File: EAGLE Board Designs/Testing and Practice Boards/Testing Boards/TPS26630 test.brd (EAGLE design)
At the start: 100 x 80 mm, 3 parts

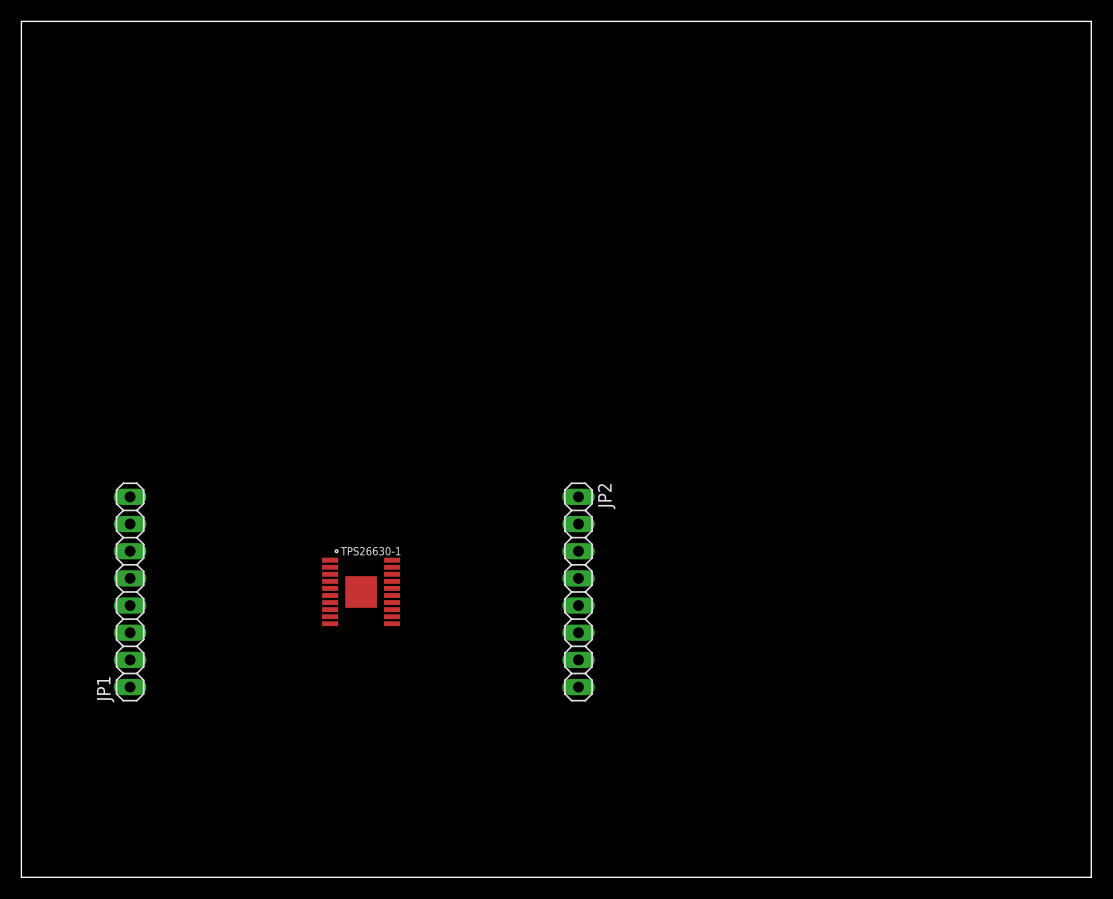
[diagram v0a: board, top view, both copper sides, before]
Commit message: Finished the TPS26630 E-Fuse breakout board layout
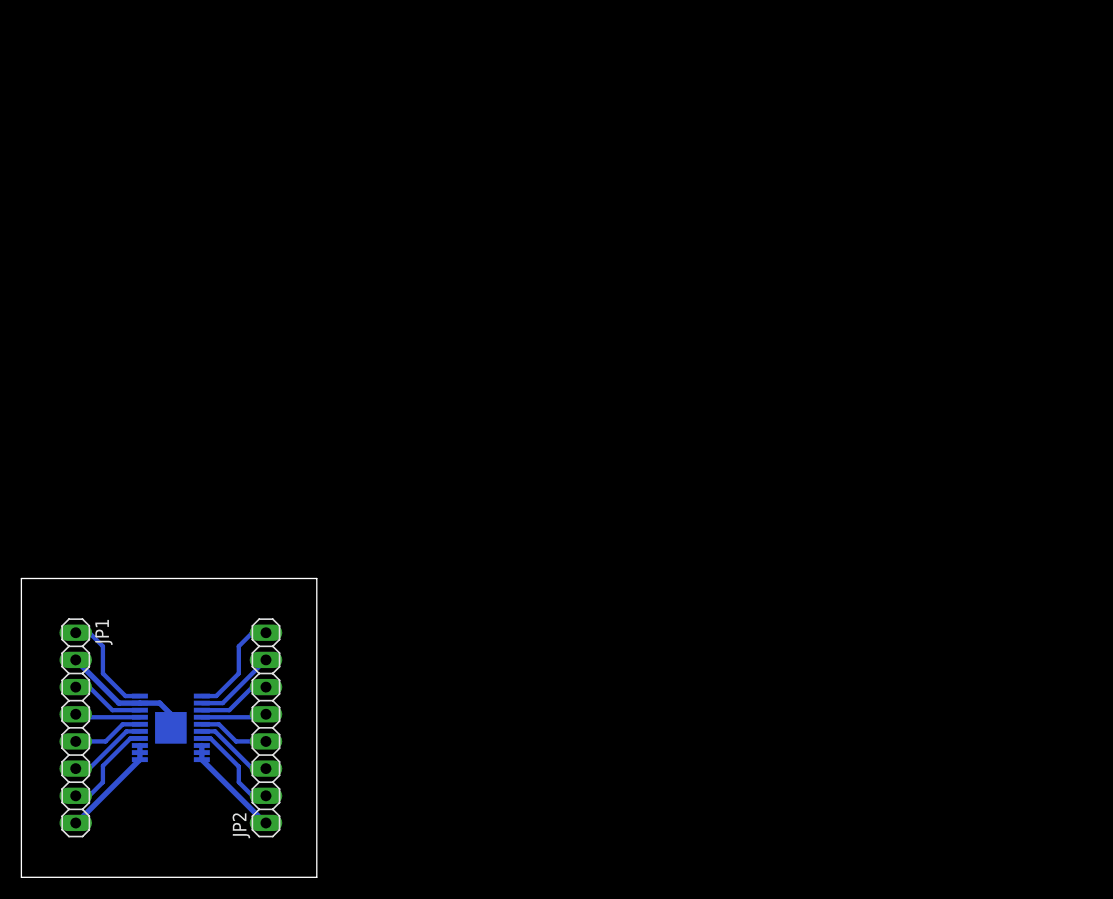
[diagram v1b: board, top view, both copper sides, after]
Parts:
- moved JP2 31.9 mm to (22.9, 14.0), turned to 90 degrees
- moved TPS26630-1 21.8 mm to (14.0, 14.0), flipped to the bottom, turned to 180 degrees
- moved JP1 13.7 mm to (5.08, 14.0), turned to 270 degrees
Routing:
- net GND: track 0.00 -> 12.3 mm
- net ILIM: track 0.00 -> 9.93 mm
- net DVDT: track 0.00 -> 9.93 mm
- net IN: track 0.00 -> 9.77 mm
- net OUT: track 0.00 -> 9.77 mm
- net B_GATE: track 0.00 -> 9.11 mm
- net PGOOD: track 0.00 -> 9.07 mm
- net MODE: track 0.00 -> 7.67 mm
- net DRV: track 0.00 -> 7.44 mm
- net PGTH: track 0.00 -> 7.44 mm
- net OVP: track 0.00 -> 6.89 mm
- net SHDN: track 0.00 -> 6.89 mm
- net IN_SYS: track 0.00 -> 6.66 mm
- net FLT: track 0.00 -> 6.66 mm
- net UVLO: track 0.00 -> 6.11 mm
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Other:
- board size 100 x 80 mm -> 27.6 x 27.9 mm
